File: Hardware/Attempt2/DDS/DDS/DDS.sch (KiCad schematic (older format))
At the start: 20 parts, among them J1 Conn_01x04_Male, J2 Conn_01x02_Male, U1 74LVC2T45DC, U2 74LVC2T45DC, U3 AD9835, X1 50MHz

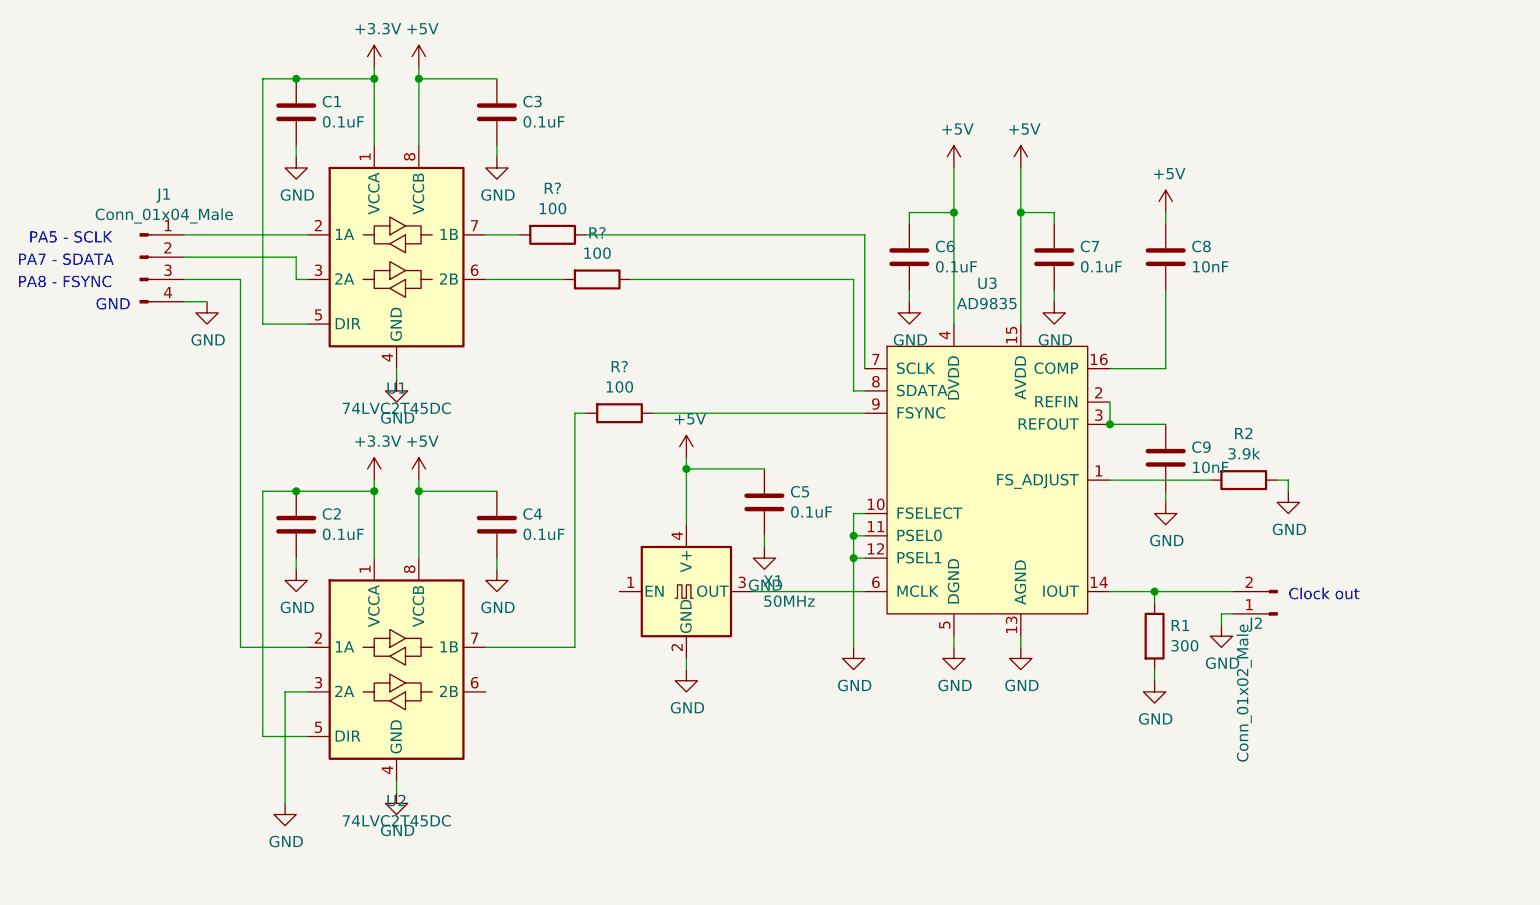
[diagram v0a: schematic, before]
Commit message: Committing forgotten changes
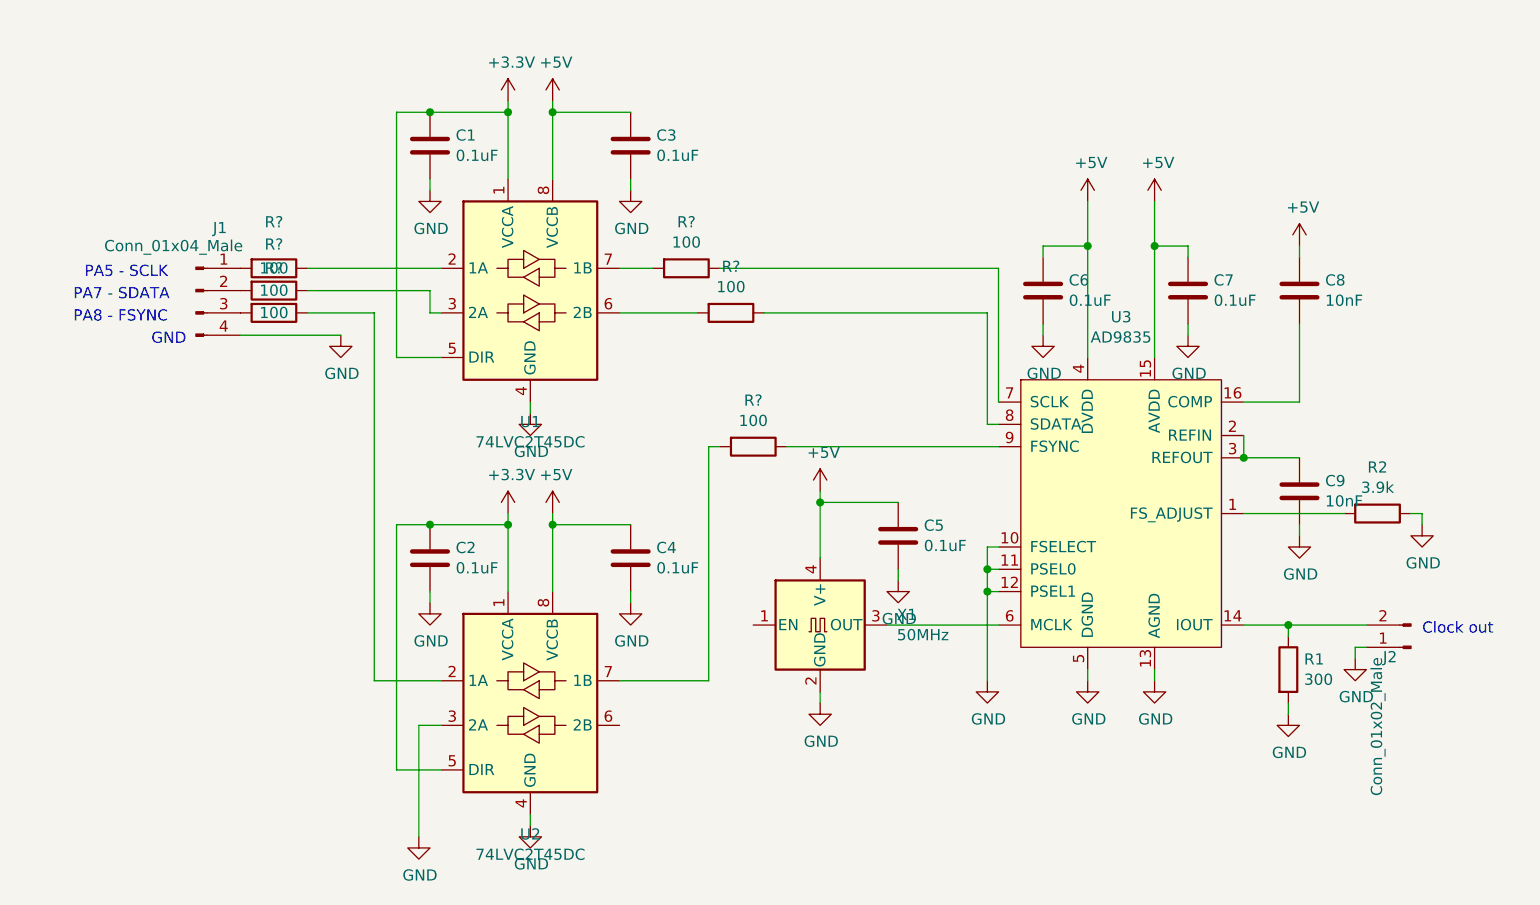
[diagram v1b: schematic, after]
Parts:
- added R? (x3): 100, symbol Device:R
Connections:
- net at U1.2 (1A): now also R?.1; no longer J1.1 (Pin_1)
- net at U1.3 (2A): now also R?.1; no longer J1.2 (Pin_2)
- net at U2.2 (1A): now also R?.1; no longer J1.3 (Pin_3)
- new net: J1.1 (Pin_1), R?.2
- new net: J1.2 (Pin_2), R?.2
- new net: J1.3 (Pin_3), R?.2
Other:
- moved on the sheet: C1, C2, C3, C4, C5, C6, C7, C8, C9, J1, J2, R1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
